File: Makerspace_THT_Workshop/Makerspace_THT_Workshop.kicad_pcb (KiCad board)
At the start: 2 copper layers, 123.3 x 94.8 mm, 22 parts, among them SW1 SW_SPDT, U1 LM358, U2 LMC555xN

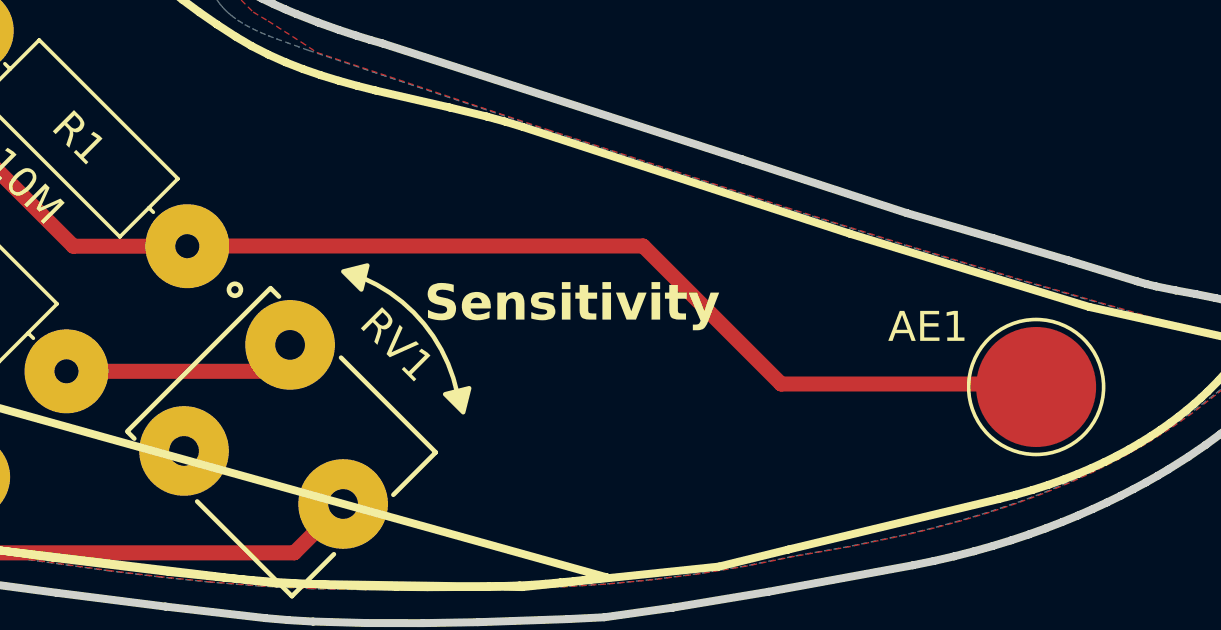
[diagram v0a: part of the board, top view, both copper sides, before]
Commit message: Minor Layout Changes
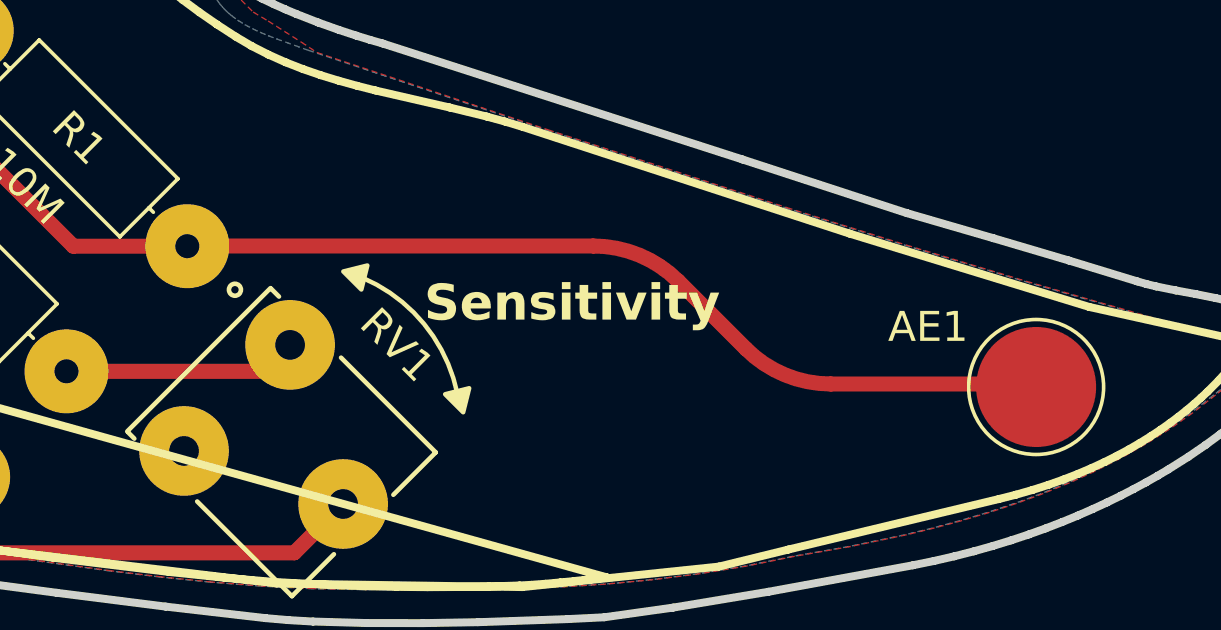
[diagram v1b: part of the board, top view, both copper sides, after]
